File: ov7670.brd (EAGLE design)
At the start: 50.8 x 42.2 mm, 3 parts

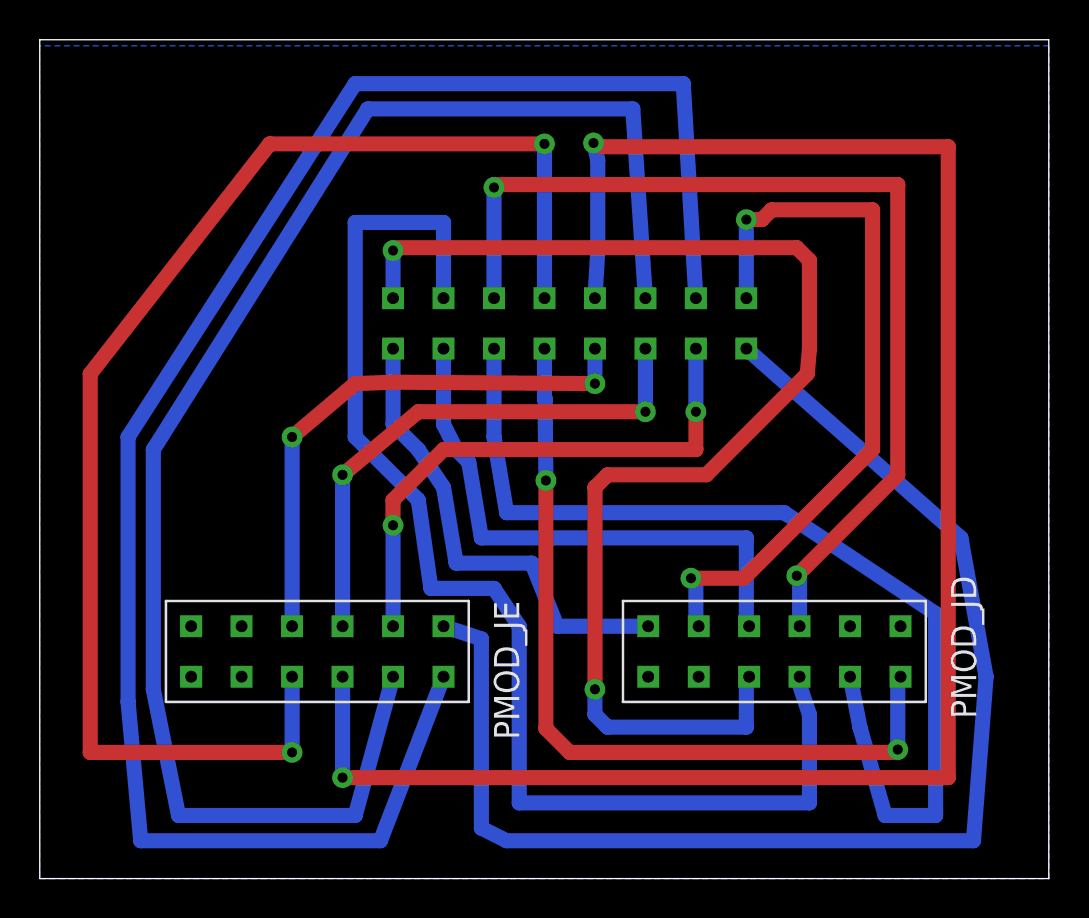
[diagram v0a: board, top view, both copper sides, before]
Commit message: update design
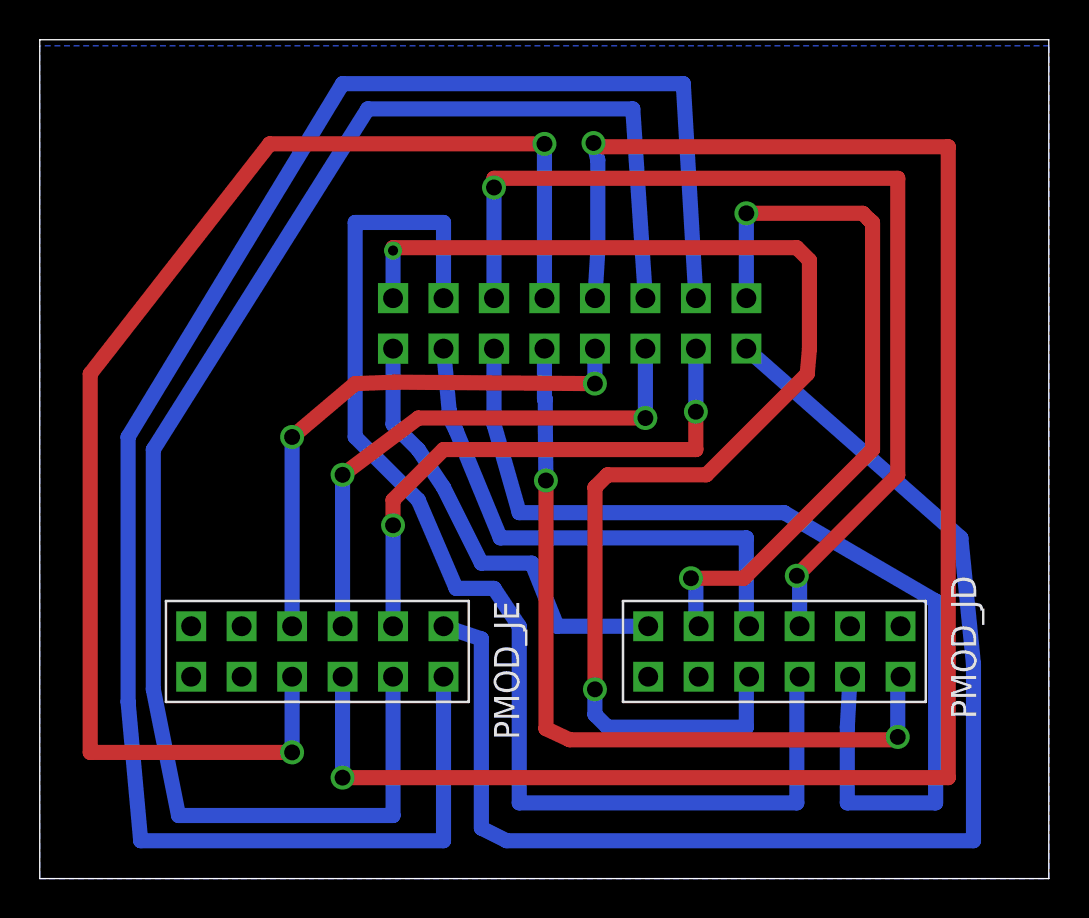
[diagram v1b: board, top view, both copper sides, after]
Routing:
- net D6: track 89.7 -> 92.6 mm
- net PLCK: track 63.6 -> 61.9 mm
- net D4: track 77.8 -> 79.5 mm
- net SDA: track 41.2 -> 40.2 mm
- net 3V3: track 23.6 -> 22.7 mm
- net SCL: track 50.4 -> 51.1 mm
- net VSYNC: track 27.9 -> 27.3 mm

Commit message: update
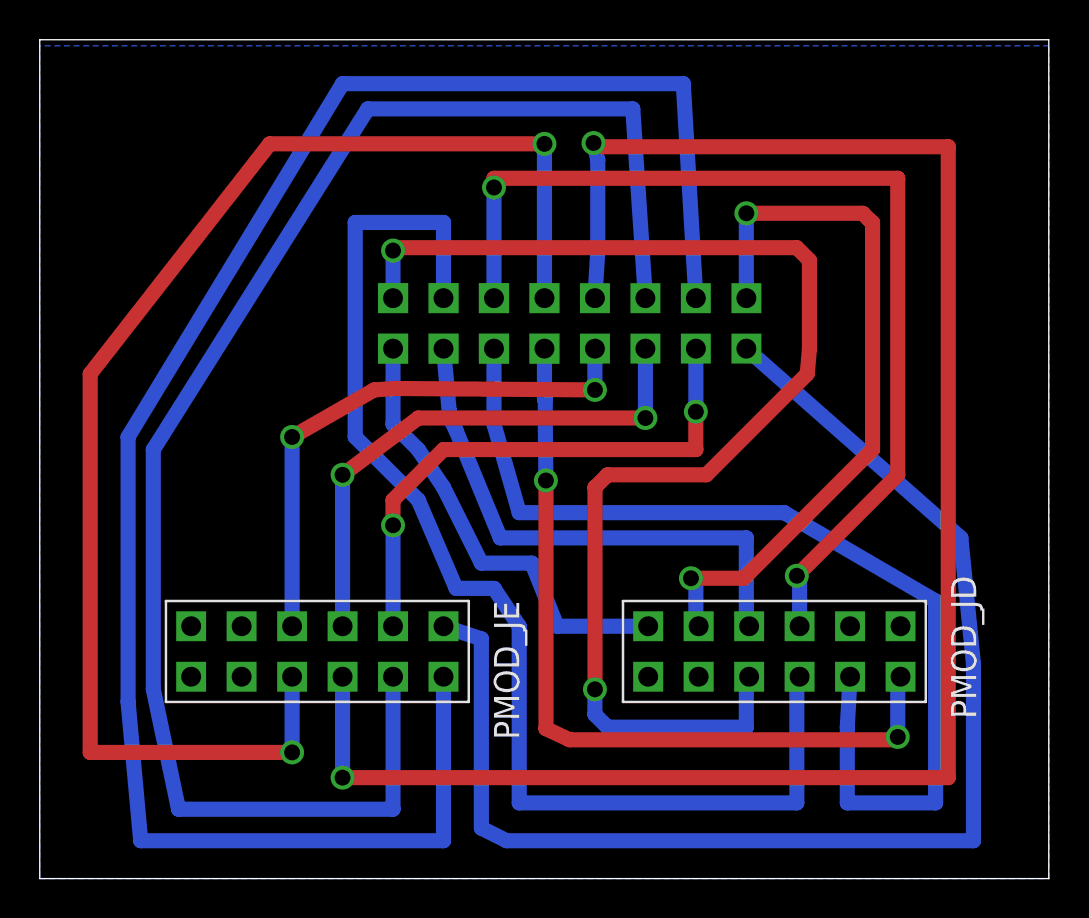
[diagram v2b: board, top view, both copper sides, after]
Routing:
- net D4: track 79.5 -> 78.8 mm
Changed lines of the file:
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@@
 <wire x1="38.735" y1="31.115" x2="38.1" y2="31.75" width="0.762" layer="1"/>
 <wire x1="17.78" y1="31.75" x2="17.78" y2="31.606" width="0.762" layer="1"/>
-<via x="17.78" y="31.606" extent="1-16" drill="0.508" diameter="0.8"/>
+<via x="17.78" y="31.606" extent="1-16" drill="0.8" diameter="0.8"/>
 <wire x1="17.78" y1="31.606" x2="17.78" y2="29.21" width="0.762" layer="16"/>
 <wire x1="38.1" y1="31.75" x2="17.78" y2="31.75" width="0.762" layer="1"/>
@@
 <contactref element="U$3" pad="4"/>
 <contactref element="U$1" pad="D1"/>
-<via x="27.94" y="24.909" extent="1-16" drill="0.8" diameter="1.05"/>
-<wire x1="27.94" y1="24.909" x2="17.85346875" y2="24.98246875" width="0.762" layer="1"/>
-<wire x1="27.94" y1="26.67" x2="27.94" y2="24.909" width="0.762" layer="16"/>
-<wire x1="17.85346875" y1="24.98246875" x2="15.875" y2="24.909" width="0.762" layer="1"/>
+<via x="27.94" y="24.5915" extent="1-16" drill="0.8" diameter="1.05"/>
+<wire x1="27.94" y1="24.5915" x2="17.85346875" y2="24.66496875" width="0.762" layer="1"/>
+<wire x1="27.94" y1="26.67" x2="27.94" y2="24.5915" width="0.762" layer="16"/>
+<wire x1="17.85346875" y1="24.66496875" x2="16.8275" y2="24.5915" width="0.762" layer="1"/>
 <via x="12.7" y="22.225" extent="1-16" drill="0.8" diameter="0.8"/>
 <wire x1="12.7" y1="22.225" x2="12.7" y2="12.7" width="0.762" layer="16"/>
-<wire x1="15.875" y1="24.909" x2="12.7" y2="22.225" width="0.762" layer="1"/>
+<wire x1="16.8275" y1="24.5915" x2="12.7" y2="22.225" width="0.762" layer="1"/>
 </signal>
 <signal name="D6">
@@
 <contactref element="U$3" pad="8"/>
 <contactref element="U$1" pad="D4"/>
-<wire x1="17.78" y1="3.175" x2="17.78" y2="10.16" width="0.762" layer="16"/>
-<wire x1="6.985" y1="3.175" x2="17.78" y2="3.175" width="0.762" layer="16"/>
-<wire x1="5.715" y1="9.525" x2="6.985" y2="3.175" width="0.762" layer="16"/>
+<wire x1="17.78" y1="3.4925" x2="17.78" y2="10.16" width="0.762" layer="16"/>
+<wire x1="6.985" y1="3.4925" x2="17.78" y2="3.4925" width="0.762" layer="16"/>
+<wire x1="5.715" y1="9.525" x2="6.985" y2="3.4925" width="0.762" layer="16"/>
 <wire x1="5.715" y1="21.59" x2="5.715" y2="9.525" width="0.762" layer="16"/>
 <wire x1="16.51" y1="38.735" x2="5.715" y2="21.59" width="0.762" layer="16"/>
